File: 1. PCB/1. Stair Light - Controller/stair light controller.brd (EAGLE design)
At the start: 82.9 x 104.1 mm, 62 parts, among them IC1 ESP32-WROVER-B, IC2 CP2104, IC3 HT7333, IC4 MAX3485, IC5 DS3231, IC6 HTU21D, J2 TFT_GC9A01, Q1 MMBT2222, Q2 MMBT2222, Q3 MMBT2222, U1" ESP32-WROOM, X1 USB-C, X2 MicroSD

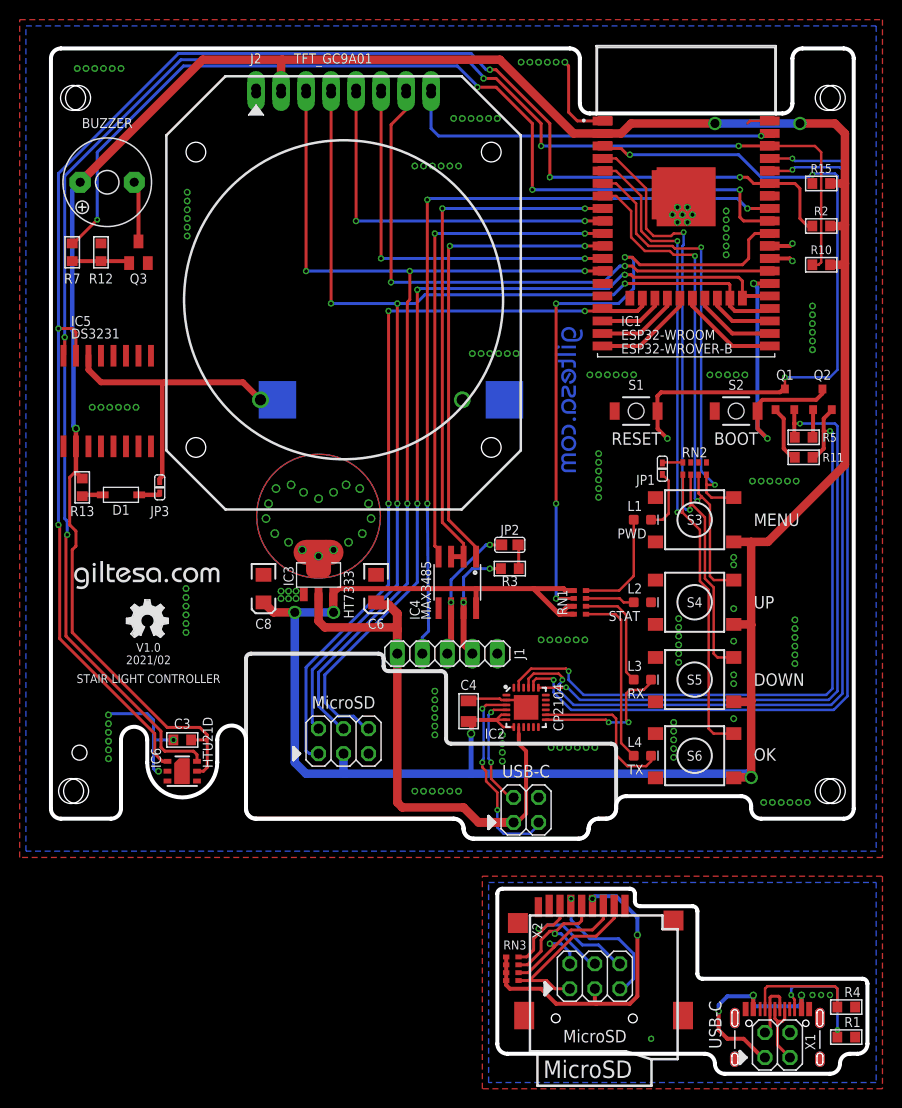
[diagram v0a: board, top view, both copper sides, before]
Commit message: Released v1.0 and sending the boards to manufacture.
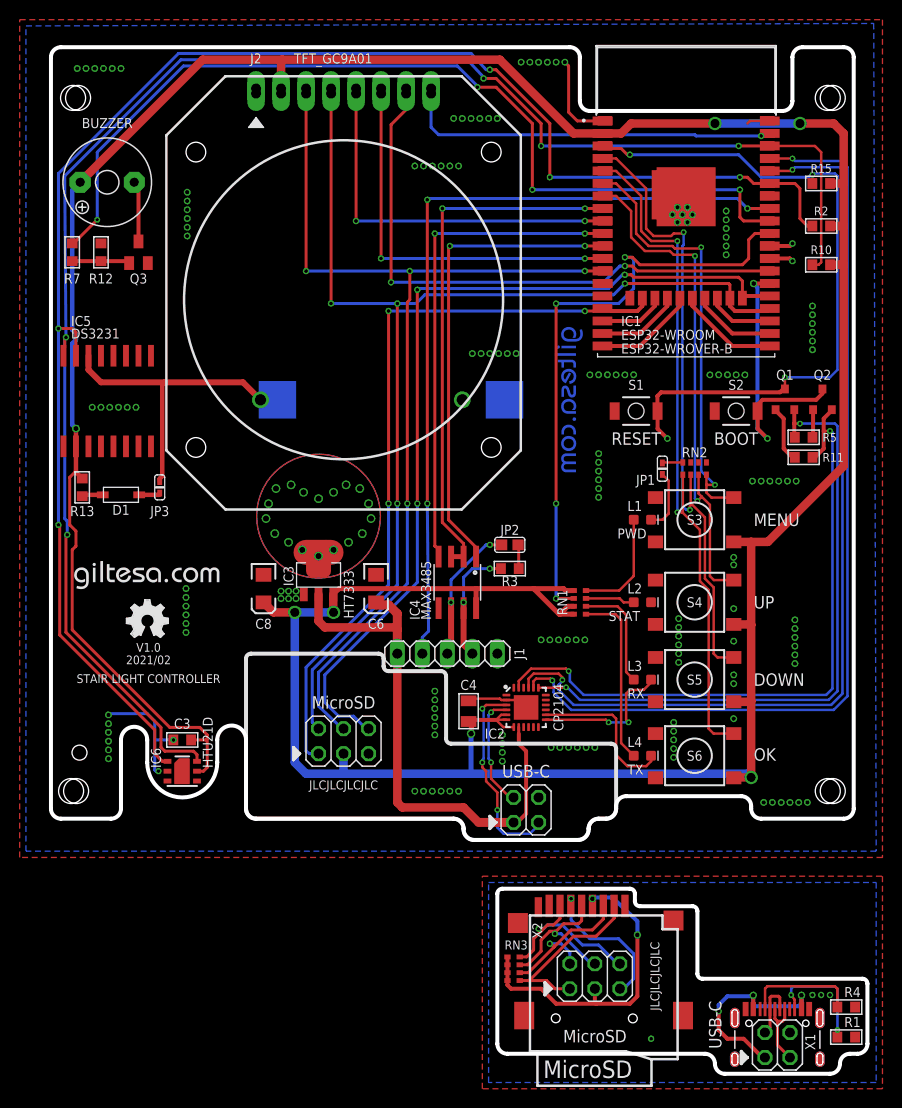
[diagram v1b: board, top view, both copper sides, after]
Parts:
- D1: value 1N4148 -> 1N4148
- moved RN3 0.13 mm to (47.0, -15.7)
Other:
- board size 82.9 x 104.1 mm -> 82.9 x 104.3 mm
- board text added: "JLCJLCJLCJLC"
